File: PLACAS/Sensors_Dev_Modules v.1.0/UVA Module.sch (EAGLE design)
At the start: 5 parts

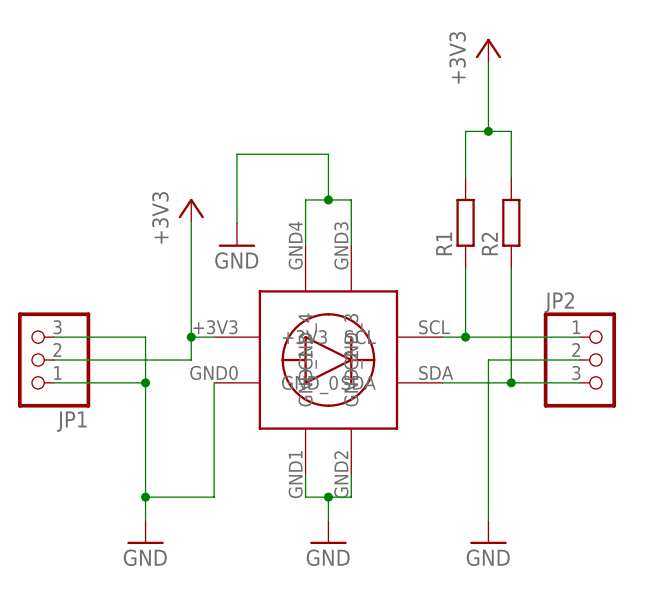
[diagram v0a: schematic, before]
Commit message: Add files via upload
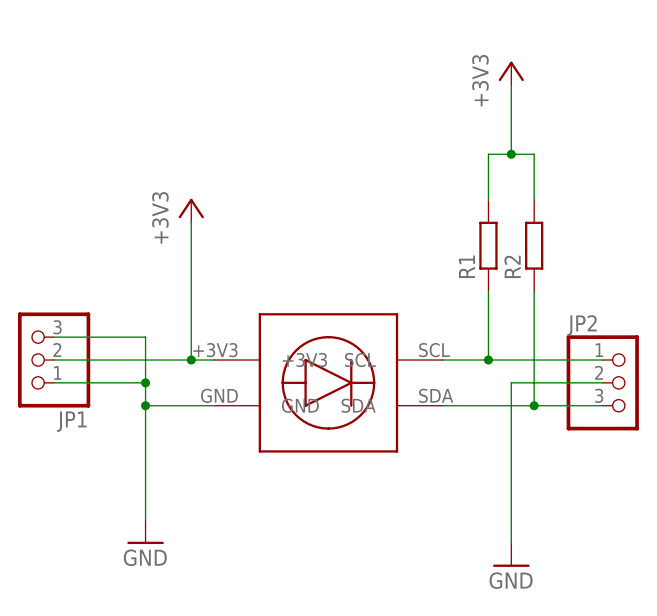
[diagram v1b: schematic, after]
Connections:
- net GND: now also U$1.GND; no longer U$1.GND_0, U$1.GND_1, U$1.GND_2, U$1.GND_3, U$1.GND_4
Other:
- moved on the sheet: JP2, R1, R2
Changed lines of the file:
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@@
 <part name="JP1" library="pinhead(1x3)" deviceset="PINHD-1X3" device="" package3d_urn="urn:adsk.eagle:package:22458/2"/>
 <part name="JP2" library="pinhead(1x3)" deviceset="PINHD-1X3" device="" package3d_urn="urn:adsk.eagle:package:22458/2"/>
-<part name="GND1" library="supply1" library_urn="urn:adsk.eagle:library:371" deviceset="GND" device=""/>
-<part name="U$1" library="Zenith_Breakouts" deviceset="BREAKOUT_UV-A" device=""/>
 <part name="GND2" library="supply1" library_urn="urn:adsk.eagle:library:371" deviceset="GND" device=""/>
 <part name="GND3" library="supply1" library_urn="urn:adsk.eagle:library:371" deviceset="GND" device=""/>
@@
 <part name="+3V1" library="supply1" library_urn="urn:adsk.eagle:library:371" deviceset="+3V3" device=""/>
 <part name="+3V2" library="supply1" library_urn="urn:adsk.eagle:library:371" deviceset="+3V3" device=""/>
-<part name="GND4" library="supply1" library_urn="urn:adsk.eagle:library:371" deviceset="GND" device=""/>
+<part name="U$1" library="Zenith_Breakouts" deviceset="BREAKOUT_UV-A" device=""/>
 </parts>
 <sheets>
@@
 <attribute name="VALUE" x="21.59" y="48.26" size="1.778" layer="96" rot="R180"/>
 </instance>
-<instance part="JP2" gate="A" x="78.74" y="40.64" smashed="yes">
-<attribute name="NAME" x="72.39" y="46.355" size="1.778" layer="95"/>
-<attribute name="VALUE" x="72.39" y="33.02" size="1.778" layer="96"/>
+<instance part="JP2" gate="A" x="81.28" y="38.1" smashed="yes">
+<attribute name="NAME" x="74.93" y="43.815" size="1.778" layer="95"/>
+<attribute name="VALUE" x="74.93" y="30.48" size="1.778" layer="96"/>
 </instance>
-<instance part="GND1" gate="1" x="48.26" y="20.32" smashed="yes">
-<attribute name="VALUE" x="45.72" y="17.78" size="1.778" layer="96"/>
-</instance>
-<instance part="U$1" gate="G$1" x="38.1" y="38.1" smashed="yes"/>
 <instance part="GND2" gate="1" x="27.94" y="20.32" smashed="yes">
 <attribute name="VALUE" x="25.4" y="17.78" size="1.778" layer="96"/>
 </instance>
-<instance part="GND3" gate="1" x="66.04" y="20.32" smashed="yes">
-<attribute name="VALUE" x="63.5" y="17.78" size="1.778" layer="96"/>
+<instance part="GND3" gate="1" x="68.58" y="17.78" smashed="yes">
+<attribute name="VALUE" x="66.04" y="15.24" size="1.778" layer="96"/>
 </instance>
-<instance part="R1" gate="G$1" x="63.5" y="55.88" smashed="yes" rot="R90">
-<attribute name="NAME" x="62.0014" y="52.07" size="1.778" layer="95" rot="R90"/>
-<attribute name="VALUE" x="66.802" y="52.07" size="1.778" layer="96" rot="R90"/>
+<instance part="R1" gate="G$1" x="66.04" y="53.34" smashed="yes" rot="R90">
+<attribute name="NAME" x="64.5414" y="49.53" size="1.778" layer="95" rot="R90"/>
+<attribute name="VALUE" x="69.342" y="49.53" size="1.778" layer="96" rot="R90"/>
 </instance>
-<instance part="R2" gate="G$1" x="68.58" y="55.88" smashed="yes" rot="R90">
-<attribute name="NAME" x="67.0814" y="52.07" size="1.778" layer="95" rot="R90"/>
-<attribute name="VALUE" x="71.882" y="52.07" size="1.778" layer="96" rot="R90"/>
+<instance part="R2" gate="G$1" x="71.12" y="53.34" smashed="yes" rot="R90">
+<attribute name="NAME" x="69.6214" y="49.53" size="1.778" layer="95" rot="R90"/>
+<attribute name="VALUE" x="74.422" y="49.53" size="1.778" layer="96" rot="R90"/>
 </instance>
-<instance part="+3V1" gate="G$1" x="66.04" y="76.2" smashed="yes">
-<attribute name="VALUE" x="63.5" y="71.12" size="1.778" layer="96" rot="R90"/>
+<instance part="+3V1" gate="G$1" x="68.58" y="73.66" smashed="yes">
+<attribute name="VALUE" x="66.04" y="68.58" size="1.778" layer="96" rot="R90"/>
 </instance>
 <instance part="+3V2" gate="G$1" x="33.02" y="58.42" smashed="yes">
 <attribute name="VALUE" x="30.48" y="53.34" size="1.778" layer="96" rot="R90"/>
 </instance>
-<instance part="GND4" gate="1" x="38.1" y="53.34" smashed="yes">
-<attribute name="VALUE" x="35.56" y="50.8" size="1.778" layer="96"/>
-</instance>
+<instance part="U$1" gate="G$1" x="38.1" y="35.56" smashed="yes"/>
 </instances>
 <busses>
@@
 <pinref part="GND2" gate="1" pin="GND"/>
 <pinref part="JP1" gate="A" pin="1"/>
-<wire x1="27.94" y1="22.86" x2="27.94" y2="25.4" width="0.1524" layer="91"/>
-<wire x1="27.94" y1="25.4" x2="27.94" y2="38.1" width="0.1524" layer="91"/>
+<wire x1="27.94" y1="22.86" x2="27.94" y2="35.56" width="0.1524" layer="91"/>
+<wire x1="27.94" y1="35.56" x2="27.94" y2="38.1" width="0.1524" layer="91"/>
 <wire x1="27.94" y1="38.1" x2="17.78" y2="38.1" width="0.1524" layer="91"/>
 <pinref part="JP1" gate="A" pin="3"/>
@@
 <wire x1="27.94" y1="43.18" x2="27.94" y2="38.1" width="0.1524" layer="91"/>
 <junction x="27.94" y="38.1"/>
-<pinref part="U$1" gate="G$1" pin="GND_0"/>
-<wire x1="35.56" y1="38.1" x2="35.56" y2="25.4" width="0.1524" layer="91"/>
-<wire x1="35.56" y1="25.4" x2="27.94" y2="25.4" width="0.1524" layer="91"/>
-<junction x="27.94" y="25.4"/>
-</segment>
-<segment>
-<pinref part="U$1" gate="G$1" pin="GND_1"/>
-<wire x1="45.72" y1="27.94" x2="45.72" y2="25.4" width="0.1524" layer="91"/>
-<wire x1="45.72" y1="25.4" x2="48.26" y2="25.4" width="0.1524" layer="91"/>
-<pinref part="U$1" gate="G$1" pin="GND_2"/>
-<wire x1="48.26" y1="25.4" x2="50.8" y2="25.4" width="0.1524" layer="91"/>
-<wire x1="50.8" y1="25.4" x2="50.8" y2="27.94" width="0.1524" layer="91"/>
-<pinref part="GND1" gate="1" pin="GND"/>
-<wire x1="48.26" y1="25.4" x2="48.26" y2="22.86" width="0.1524" layer="91"/>
-<junction x="48.26" y="25.4"/>
+<pinref part="U$1" gate="G$1" pin="GND"/>
+<wire x1="35.56" y1="35.56" x2="27.94" y2="35.56" width="0.1524" layer="91"/>
+<junction x="27.94" y="35.56"/>
 </segment>
 <segment>
 <pinref part="GND3" gate="1" pin="GND"/>
-<wire x1="66.04" y1="22.86" x2="66.04" y2="40.64" width="0.1524" layer="91"/>
+<wire x1="68.58" y1="20.32" x2="68.58" y2="38.1" width="0.1524" layer="91"/>
 <pinref part="JP2" gate="A" pin="2"/>
-<wire x1="66.04" y1="40.64" x2="76.2" y2="40.64" width="0.1524" layer="91"/>
-</segment>
-<segment>
-<pinref part="GND4" gate="1" pin="GND"/>
-<wire x1="38.1" y1="55.88" x2="38.1" y2="63.5" width="0.1524" layer="91"/>
-<wire x1="38.1" y1="63.5" x2="48.26" y2="63.5" width="0.1524" layer="91"/>
-<pinref part="U$1" gate="G$1" pin="GND_4"/>
-<wire x1="45.72" y1="53.34" x2="45.72" y2="58.42" width="0.1524" layer="91"/>
-<wire x1="45.72" y1="58.42" x2="48.26" y2="58.42" width="0.1524" layer="91"/>
-<pinref part="U$1" gate="G$1" pin="GND_3"/>
-<wire x1="48.26" y1="58.42" x2="50.8" y2="58.42" width="0.1524" layer="91"/>
-<wire x1="50.8" y1="58.42" x2="50.8" y2="53.34" width="0.1524" layer="91"/>
-<wire x1="48.26" y1="63.5" x2="48.26" y2="58.42" width="0.1524" layer="91"/>
-<junction x="48.26" y="58.42"/>
+<wire x1="68.58" y1="38.1" x2="78.74" y2="38.1" width="0.1524" layer="91"/>
 </segment>
 </net>
@@
 <segment>
 <pinref part="JP2" gate="A" pin="3"/>
+<wire x1="78.74" y1="35.56" x2="71.12" y2="35.56" width="0.1524" layer="91"/>
+<pinref part="R2" gate="G$1" pin="1"/>
+<wire x1="71.12" y1="48.26" x2="71.12" y2="35.56" width="0.1524" layer="91"/>
 <pinref part="U$1" gate="G$1" pin="SDA"/>
-<wire x1="76.2" y1="38.1" x2="68.58" y2="38.1" width="0.1524" layer="91"/>
-<pinref part="R2" gate="G$1" pin="1"/>
-<wire x1="68.58" y1="38.1" x2="60.96" y2="38.1" width="0.1524" layer="91"/>
-<wire x1="68.58" y1="50.8" x2="68.58" y2="38.1" width="0.1524" layer="91"/>
-<junction x="68.58" y="38.1"/>
+<wire x1="60.96" y1="35.56" x2="71.12" y2="35.56" width="0.1524" layer="91"/>
+<junction x="71.12" y="35.56"/>
 </segment>
 </net>
 <net name="N$5" class="0">
 <segment>
+<pinref part="JP2" gate="A" pin="1"/>
+<pinref part="R1" gate="G$1" pin="1"/>
+<wire x1="66.04" y1="40.64" x2="78.74" y2="40.64" width="0.1524" layer="91"/>
+<wire x1="66.04" y1="48.26" x2="66.04" y2="40.64" width="0.1524" layer="91"/>
 <pinref part="U$1" gate="G$1" pin="SCL"/>
-<pinref part="JP2" gate="A" pin="1"/>
-<wire x1="60.96" y1="43.18" x2="63.5" y2="43.18" width="0.1524" layer="91"/>
-<pinref part="R1" gate="G$1" pin="1"/>
-<wire x1="63.5" y1="43.18" x2="76.2" y2="43.18" width="0.1524" layer="91"/>
-<wire x1="63.5" y1="50.8" x2="63.5" y2="43.18" width="0.1524" layer="91"/>
-<junction x="63.5" y="43.18"/>
+<wire x1="60.96" y1="40.64" x2="66.04" y2="40.64" width="0.1524" layer="91"/>
+<junction x="66.04" y="40.64"/>
 </segment>
 </net>
 <net name="+3V3" class="0">
 <segment>
-<pinref part="U$1" gate="G$1" pin="+3V3"/>
-<wire x1="33.02" y1="43.18" x2="35.56" y2="43.18" width="0.1524" layer="91"/>
 <pinref part="+3V2" gate="G$1" pin="+3V3"/>
-<wire x1="33.02" y1="55.88" x2="33.02" y2="43.18" width="0.1524" layer="91"/>
+<wire x1="33.02" y1="55.88" x2="33.02" y2="40.64" width="0.1524" layer="91"/>
 <pinref part="JP1" gate="A" pin="2"/>
 <wire x1="17.78" y1="40.64" x2="33.02" y2="40.64" width="0.1524" layer="91"/>
-<wire x1="33.02" y1="40.64" x2="33.02" y2="43.18" width="0.1524" layer="91"/>
-<junction x="33.02" y="43.18"/>
+<pinref part="U$1" gate="G$1" pin="+3V3"/>
+<wire x1="33.02" y1="40.64" x2="35.56" y2="40.64" width="0.1524" layer="91"/>
+<junction x="33.02" y="40.64"/>
 </segment>
 <segment>
 <pinref part="R1" gate="G$1" pin="2"/>
-<wire x1="63.5" y1="60.96" x2="63.5" y2="66.04" width="0.1524" layer="91"/>
-<wire x1="63.5" y1="66.04" x2="66.04" y2="66.04" width="0.1524" layer="91"/>
+<wire x1="66.04" y1="58.42" x2="66.04" y2="63.5" width="0.1524" layer="91"/>
+<wire x1="66.04" y1="63.5" x2="68.58" y2="63.5" width="0.1524" layer="91"/>
 <pinref part="R2" gate="G$1" pin="2"/>
-<wire x1="66.04" y1="66.04" x2="68.58" y2="66.04" width="0.1524" layer="91"/>
-<wire x1="68.58" y1="66.04" x2="68.58" y2="60.96" width="0.1524" layer="91"/>
+<wire x1="68.58" y1="63.5" x2="71.12" y2="63.5" width="0.1524" layer="91"/>
+<wire x1="71.12" y1="63.5" x2="71.12" y2="58.42" width="0.1524" layer="91"/>
 <pinref part="+3V1" gate="G$1" pin="+3V3"/>
-<wire x1="66.04" y1="66.04" x2="66.04" y2="73.66" width="0.1524" layer="91"/>
-<junction x="66.04" y="66.04"/>
+<wire x1="68.58" y1="63.5" x2="68.58" y2="71.12" width="0.1524" layer="91"/>
+<junction x="68.58" y="63.5"/>
 </segment>
 </net>
